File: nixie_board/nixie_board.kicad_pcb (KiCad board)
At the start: 2 copper layers, 221 x 59.7 mm, 53 parts, among them J1 12V, J2 170V, J3 GND, J4 SHTDWN, U1 74LS32, U10 74LS32, U11 K155NA1, U12 L7805, U13 74HCT595, U14 K155NA1, U15 DS18B20, U2 K155NA1, U3 ESP32, U4 74HCT595, U5 K155NA1, U6 74LS32, U7 K155NA1, U8 74HCT595, U9 K155NA1

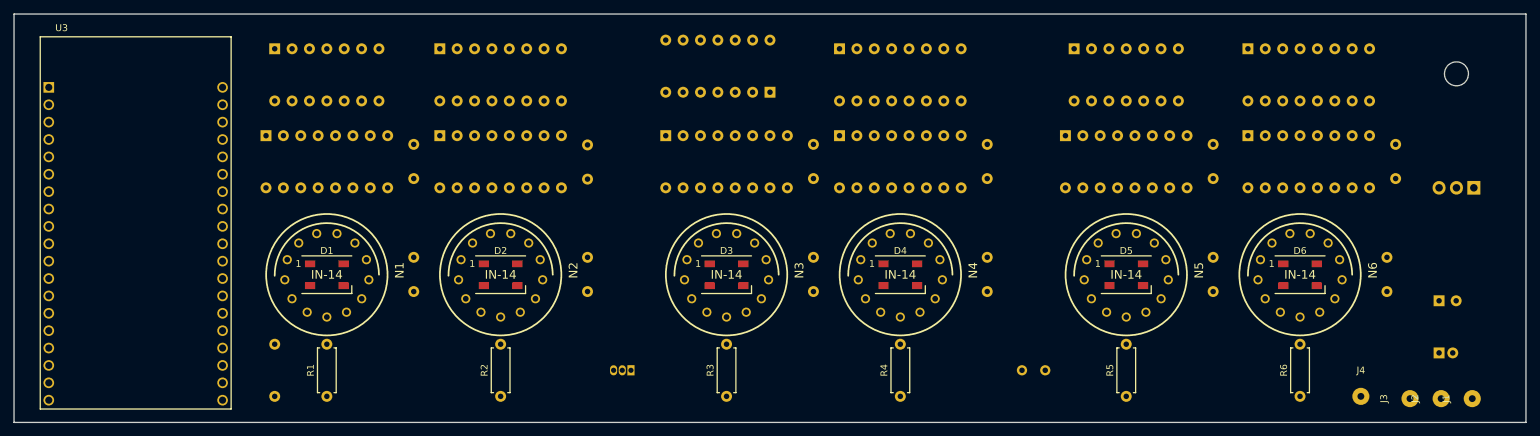
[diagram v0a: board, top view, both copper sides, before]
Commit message: rev 0.2
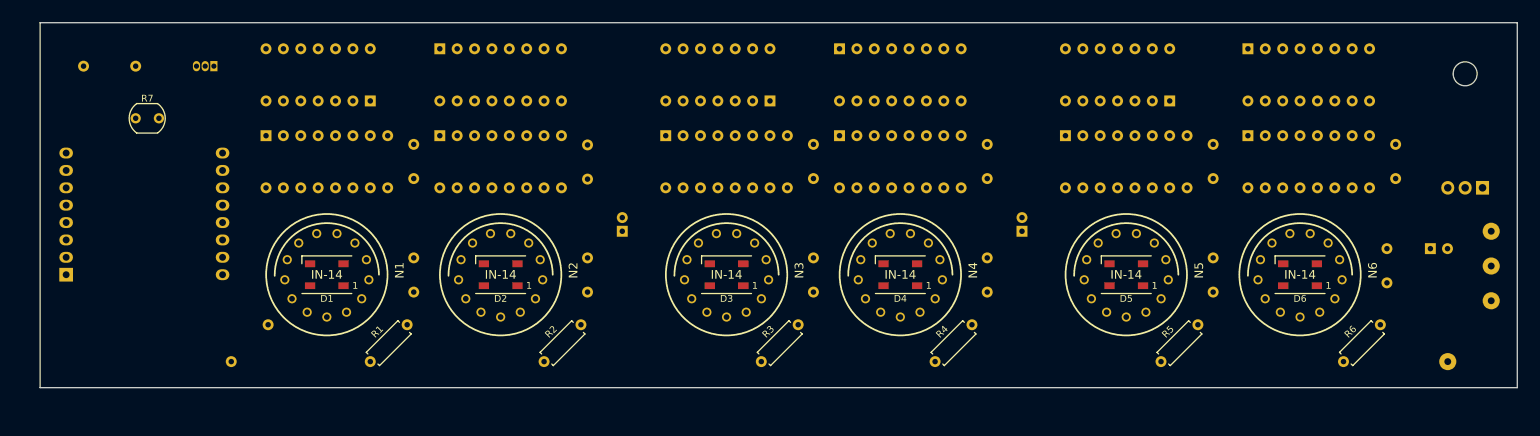
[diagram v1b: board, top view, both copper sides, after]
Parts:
- added C15: 10uF, Capacitor_THT:CP_Radial_D5.0mm_P2.00mm, B.Cu at (184.2, 50.8)
- added R9: 4.7K, Resistor_THT:R_Axial_DIN0207_L6.3mm_D2.5mm_P7.62mm_Horizontal, B.Cu at (47.0, 26.7)
- J1, J2, J3: moved to B.Cu
- J4: value SHTDWN -> SHDN; moved to B.Cu
- R7: moved to F.Cu
- U3: value ESP32 -> WeMos_D1_mini; footprint ESP32-DEVKITC-32D:MODULE_ESP32-DEVKITC-32D -> Module:WEMOS_D1_mini_light; moved to B.Cu
- moved R7 134.7 mm to (54.6, 34.3)
- moved C8 120.7 mm to (125.7, 50.8), turned to 90 degrees
- moved U15 75.4 mm to (66.0, 26.7)
- moved J1 24.6 mm to (252.7, 50.8), turned to 270 degrees
- moved J4 23.6 mm to (252.7, 61.0), turned to 270 degrees
- moved J3 22.7 mm to (252.7, 55.9), turned to 270 degrees
- moved U1 15.9 mm to (88.9, 31.8), turned to 90 degrees
- moved U10 15.9 mm to (205.7, 31.8), turned to 90 degrees
- moved U3 12.7 mm to (44.5, 57.1)
- moved R1 8.13 mm to (88.9, 69.8), turned to 45 degrees
- moved R8 8.13 mm to (68.6, 69.8), turned to 45 degrees
- moved R2 8.13 mm to (114.3, 69.8), turned to 45 degrees
- moved R6 8.13 mm to (231.1, 69.8), turned to 45 degrees
- moved C7 7.73 mm to (243.8, 53.3)
- moved R3 7.18 mm to (146.1, 69.8), turned to 45 degrees
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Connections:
- U15 pad 2: Net-(U15-Pad2) -> Net-(R9-Pad2)
- U3 pad 1: /3.3V -> (no net)
- U3 pad 10: (no net) -> GND
- U3 pad 11: (no net) -> /RCLK
- U3 pad 12: (no net) -> /SER
- U3 pad 13: (no net) -> Net-(R9-Pad2)
- U3 pad 14: GND -> (no net)
- U3 pad 2: (no net) -> Net-(R7-Pad2)
- U3 pad 4: (no net) -> /SRCLK
- U3 pad 5: (no net) -> /SHUTDOWN
- U3 pad 6: (no net) -> /RGB
- U3 pad 7: (no net) -> /STROBE
- U3 pad 8: (no net) -> /3.3V
- U3 pad 9: (no net) -> /5V
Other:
- board size 221 x 59.7 mm -> 215.9 x 53.3 mm
- net class 5v rail: clearance 0.25 -> 0.35; trace_width 0.28 -> 0.35
- net class Default: clearance 0.25 -> 0.3; trace_width 0.25 -> 0.3
- net class HighVoltage: trace_width 0.35 -> 0.5
- rule trace_clearance: 0.25 -> 0.3

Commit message: clearence review
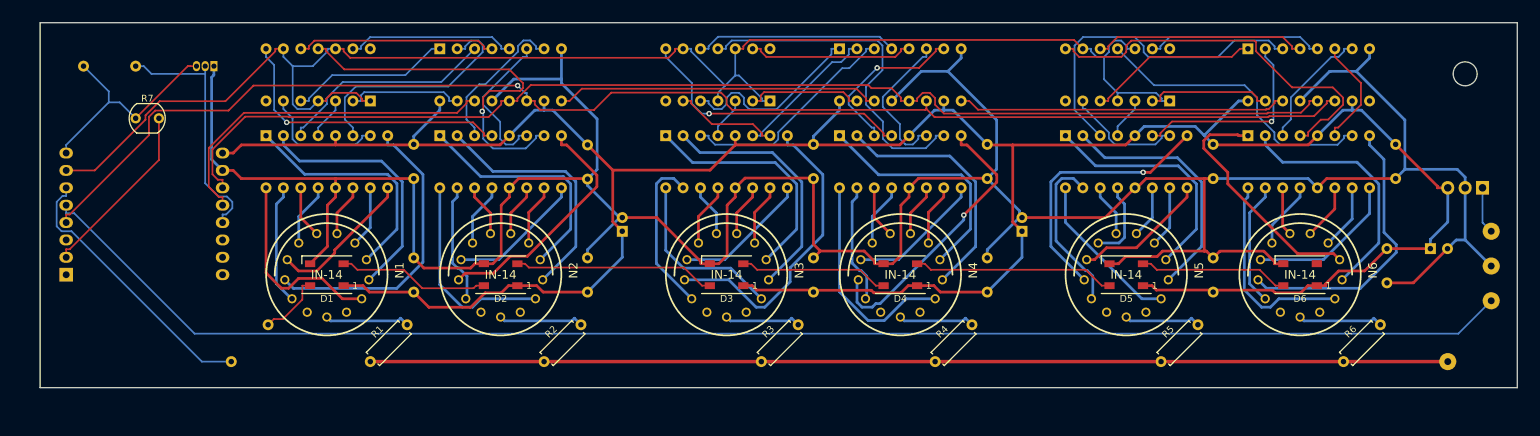
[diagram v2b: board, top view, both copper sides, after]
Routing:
- net GND: track 0.00 -> 461.9 mm
- net /5V: track 0.00 -> 407.3 mm
- net /STROBE: track 0.00 -> 224.0 mm
- net /SHUTDOWN: track 0.00 -> 218.7 mm
- net /SRCLK: track 0.00 -> 204.0 mm, vias 0 -> 1
- net /RCLK: track 0.00 -> 177.4 mm
- net /170V: track 0.00 -> 157.5 mm
- net Net-(U10-Pad8): track 0.00 -> 56.5 mm
- net Net-(U1-Pad11): track 0.00 -> 56.0 mm, vias 0 -> 1
- net /SER: track 0.00 -> 51.4 mm
- net Net-(U6-Pad11): track 0.00 -> 51.2 mm
- net Net-(U11-Pad3): track 0.00 -> 49.1 mm
- net Net-(U13-Pad14): track 0.00 -> 48.2 mm
- net Net-(U4-Pad9): track 0.00 -> 47.4 mm
- net Net-(N3-Pad2): track 0.00 -> 44.6 mm
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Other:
- net class 5v rail: trace_width 0.35 -> 0.4
- net class Default: clearance 0.3 -> 0.254; trace_width 0.3 -> 0.254
- net class HighVoltage removed
- net class HighVoltageIN added: clearance 0.35, trace_width 0.5, via_dia 0.8, via_drill 0.4
- net class HighVoltageOut added: clearance 0.35, trace_width 0.4, via_dia 0.8, via_drill 0.4
- rule trace_clearance: 0.3 -> 0.254
